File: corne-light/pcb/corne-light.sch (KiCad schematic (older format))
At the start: 72 parts, among them J1 MJ-4PP-9, J2 OLED, J6 MJ-4PP-9, J7 OLED, SW1 SW_PUSH, SW10 SW_PUSH, SW11 SW_PUSH, SW12 SW_PUSH, SW13 SW_PUSH, SW14 SW_PUSH, SW15 SW_PUSH, SW16 SW_PUSH, SW17 SW_PUSH, SW18 SW_PUSH, SW19 SW_PUSH, SW2 SW_PUSH, SW20 SW_PUSH, SW21 SW_PUSH, SW22 SW_PUSH, SW23 SW_PUSH, SW24 SW_PUSH, SW25 SW_PUSH, SW26 SW_PUSH, SW27 SW_PUSH, SW28 SW_PUSH, SW29 SW_PUSH, SW3 SW_PUSH, SW30 SW_PUSH, SW31 SW_PUSH, SW32 SW_PUSH, SW33 SW_PUSH, SW34 SW_PUSH, SW35 SW_PUSH, SW36 SW_PUSH, SW37 SW_PUSH, SW38 SW_PUSH, SW39 SW_PUSH, SW4 SW_PUSH, SW40 SW_PUSH, SW41 SW_PUSH, SW42 SW_PUSH, SW5 SW_PUSH, SW6 SW_PUSH, SW7 SW_PUSH, SW8 SW_PUSH, SW9 SW_PUSH, U1 ProMicro, U2 ProMicro

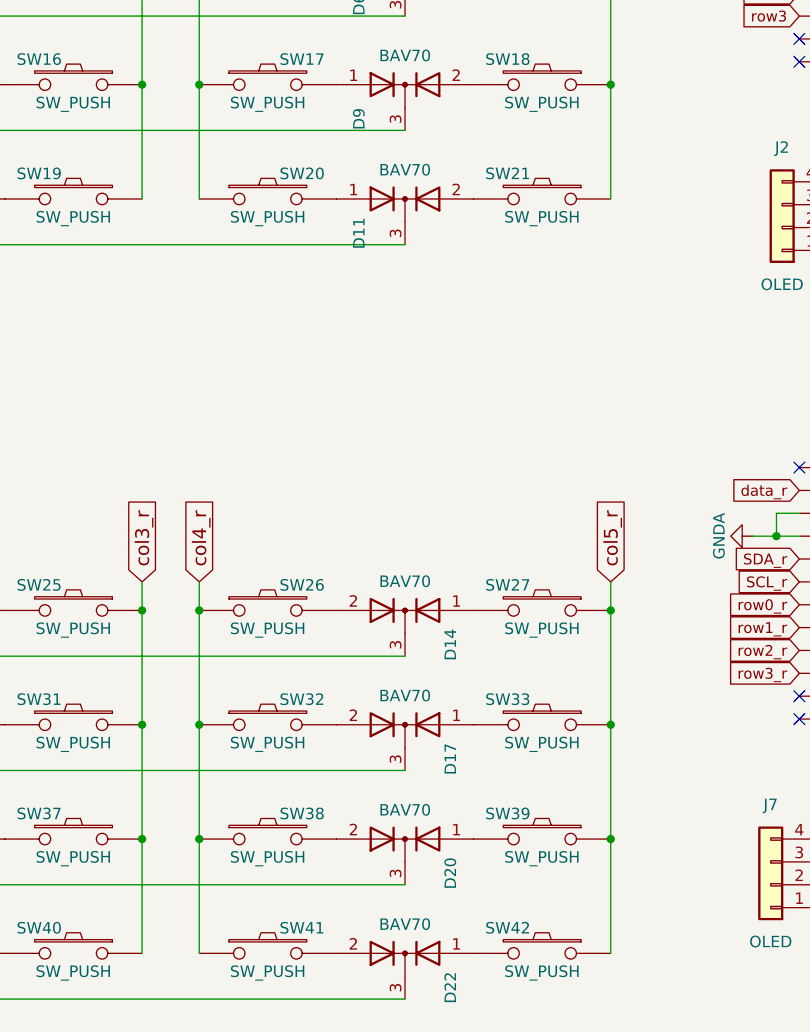
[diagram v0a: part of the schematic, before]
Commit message: Route mcu
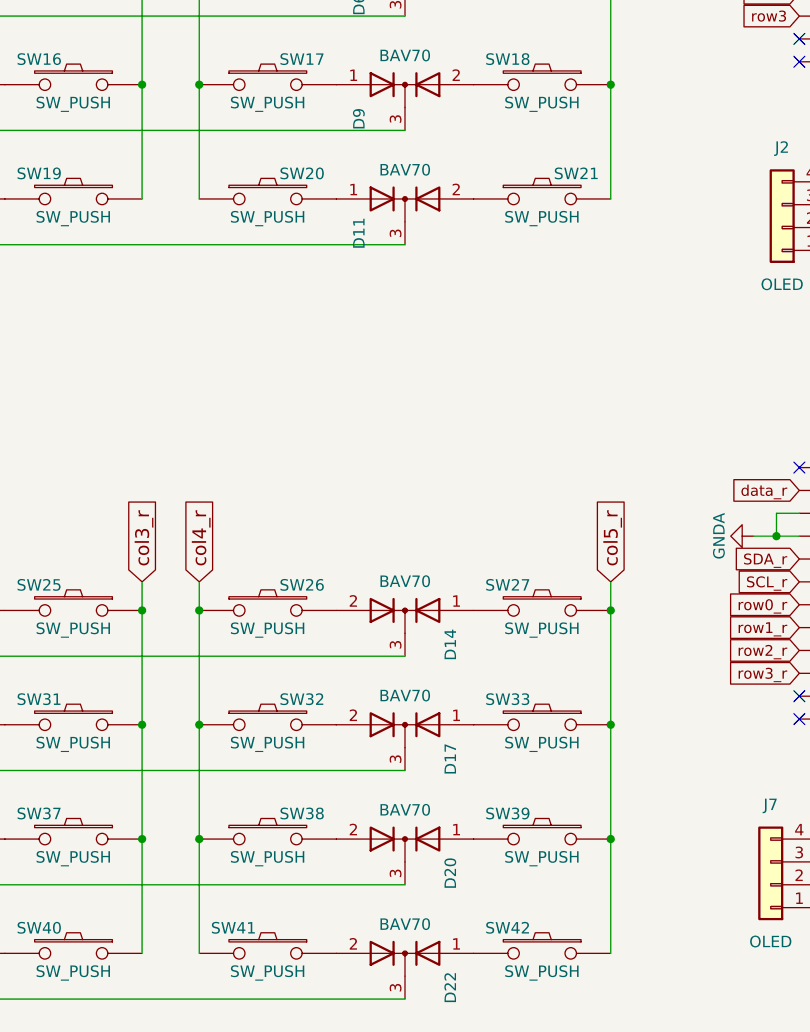
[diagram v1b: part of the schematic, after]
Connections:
- net col4_r: now also SW41.2; no longer SW41.1
- net col5: now also SW21.2; no longer SW21.1
- net at D11.2 (A): now also SW21.1; no longer SW21.2
- net at D22.2 (A): now also SW41.1; no longer SW41.2
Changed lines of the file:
@@
 F 3 "" H 6550 2725 50  0000 C CNN
 	1    6550 2725
-	-1   0    0    -1
+	1    0    0    -1
 $EndComp
 $Comp
@@
 F 3 "" H 5350 6025 50  0000 C CNN
 	1    5350 6025
-	1    0    0    -1
-$EndComp
-$Comp
+	-1   0    0    -1
+$EndComp
+$Comp
